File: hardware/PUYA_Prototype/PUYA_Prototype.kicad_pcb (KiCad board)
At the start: 2 copper layers, 19.3 x 31.8 mm, 26 parts, among them J1 SWD, J2 L_Terminal, J3 R_Terminal, SW1 SW_RST, U1 PY32F002AA15M6TU, U2 AP2112K-3.3TRG1

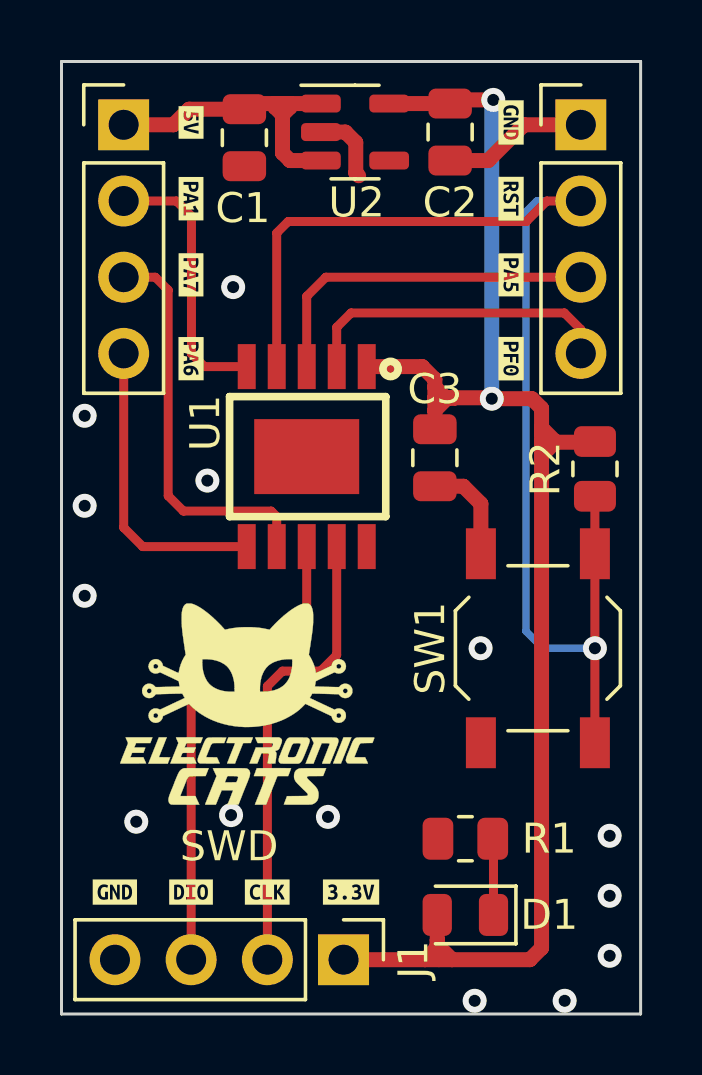
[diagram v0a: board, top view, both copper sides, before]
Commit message: fix library
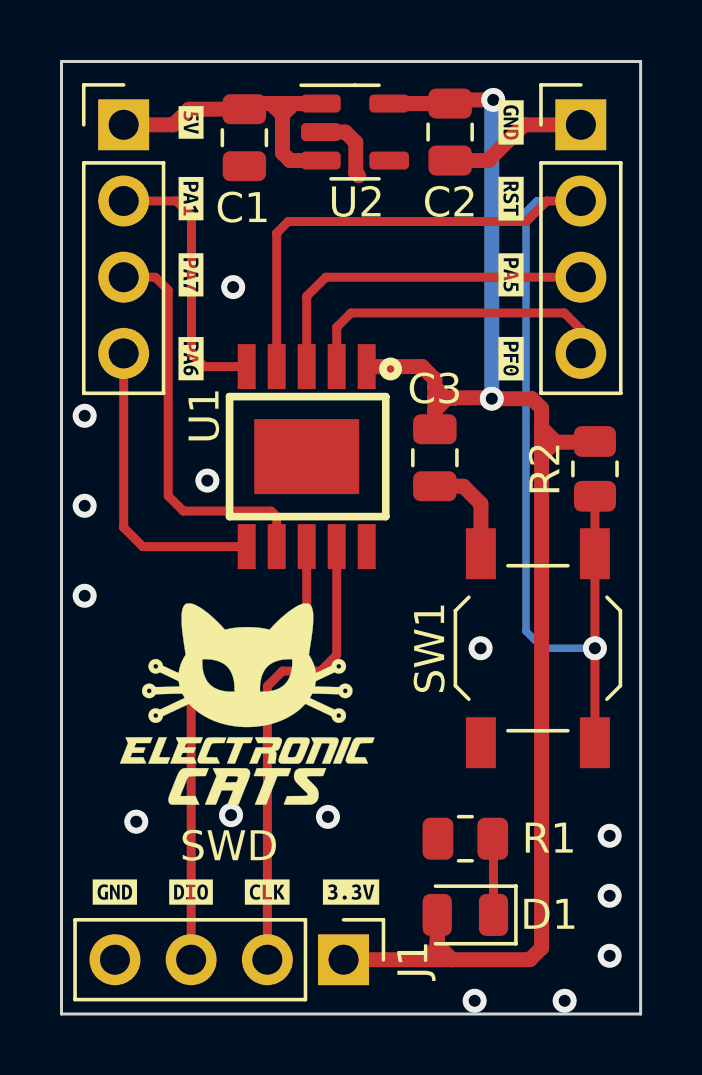
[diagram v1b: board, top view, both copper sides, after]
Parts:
- U1: footprint PY32F002:PY32F002AA15M -> Librarie:PY32F002AA15M
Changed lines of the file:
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@@
       (stroke (width 0) (type solid)) (fill solid) (layer "F.SilkS"))
   )
-  (footprint "PY32F002:PY32F002AA15M" (layer "F.Cu")
+  (footprint "Librarie:PY32F002AA15M" (layer "F.Cu")
     (at 117.902002 72.859873 -90)
     (property "LCSC#" "C5292058")
@@
     (property "manf#" "")
     (attr through_hole)
-    (fp_text reference "U1" (at -1.119873 3.382002 90) (layer "F.SilkS")
+    (fp_text reference "U1" (at -1.359873 3.402002 -90) (layer "F.SilkS")
         (effects (font (size 1 1) (thickness 0.15)))
     )
-    (fp_text value "PY32F002AA15M6TU" (at 0 3.5 90) (layer "F.Fab")
+    (fp_text value "PY32F002AA15M6TU" (at 0 3.5 -90) (layer "F.Fab")
         (effects (font (size 1 1) (thickness 0.15)))
     )
